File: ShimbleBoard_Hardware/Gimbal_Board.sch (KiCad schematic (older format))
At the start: 54 parts, among them Q1 2N3904, Q2 2N3904, Q3 2N3904, Q4 2N3904, Q5 2N3904, Q6 2N3904, Q7 2N3904, Q8 2N3904, U1 TM4C129E_Launchpad, U2 OKI, U3 OKI

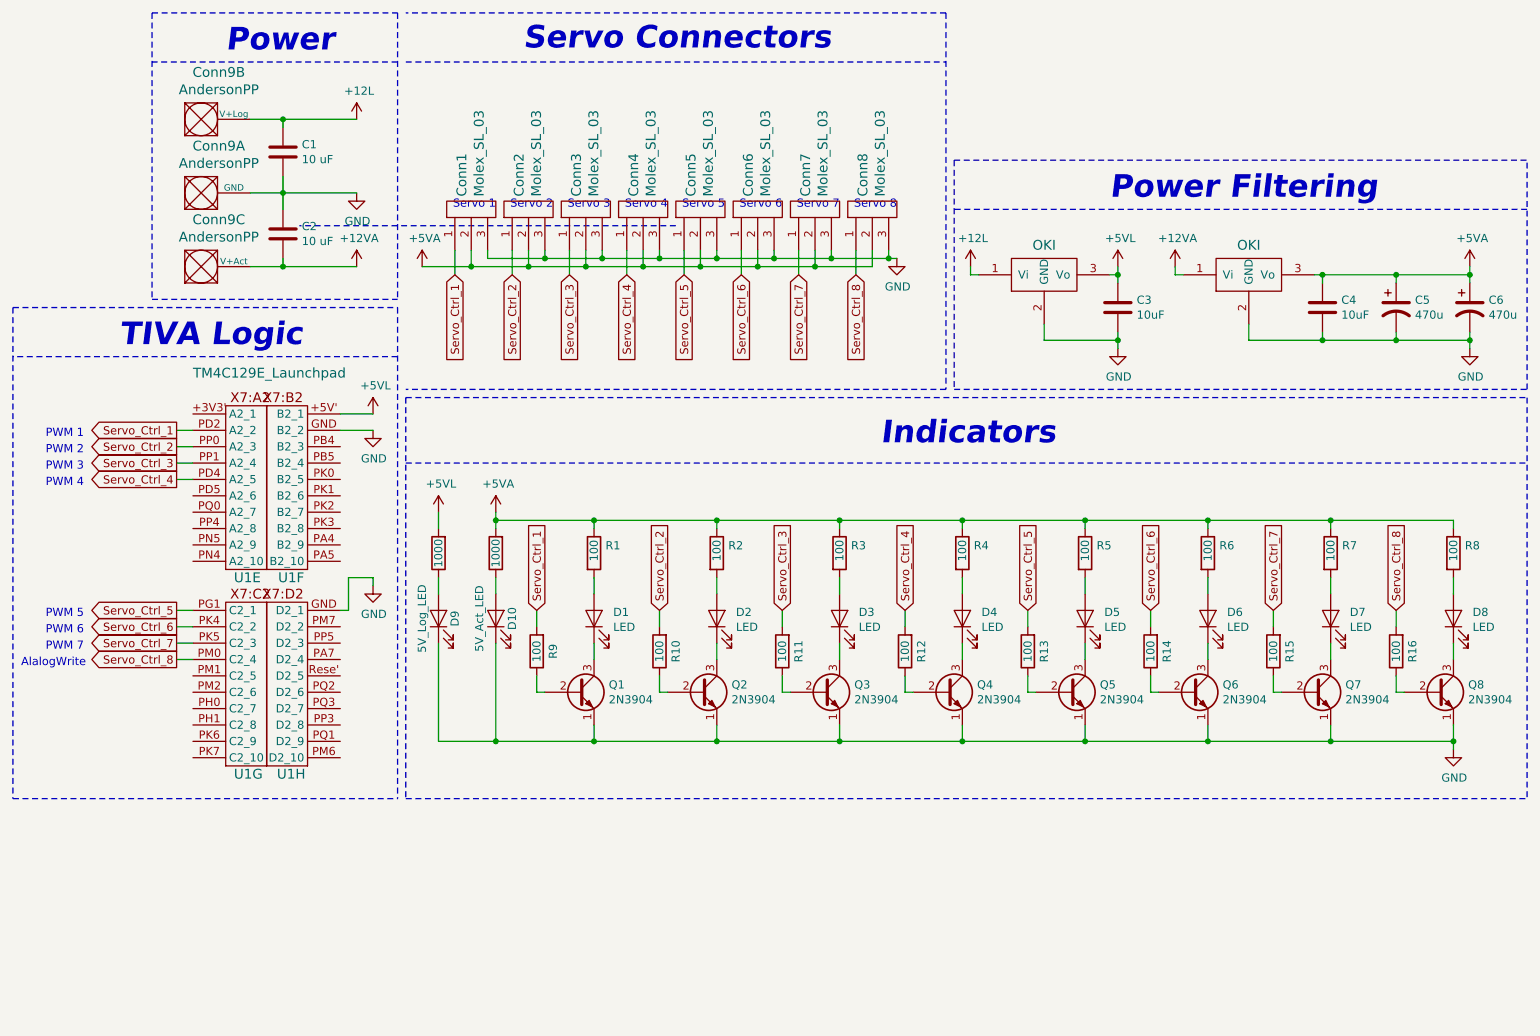
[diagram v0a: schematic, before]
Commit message: Noice
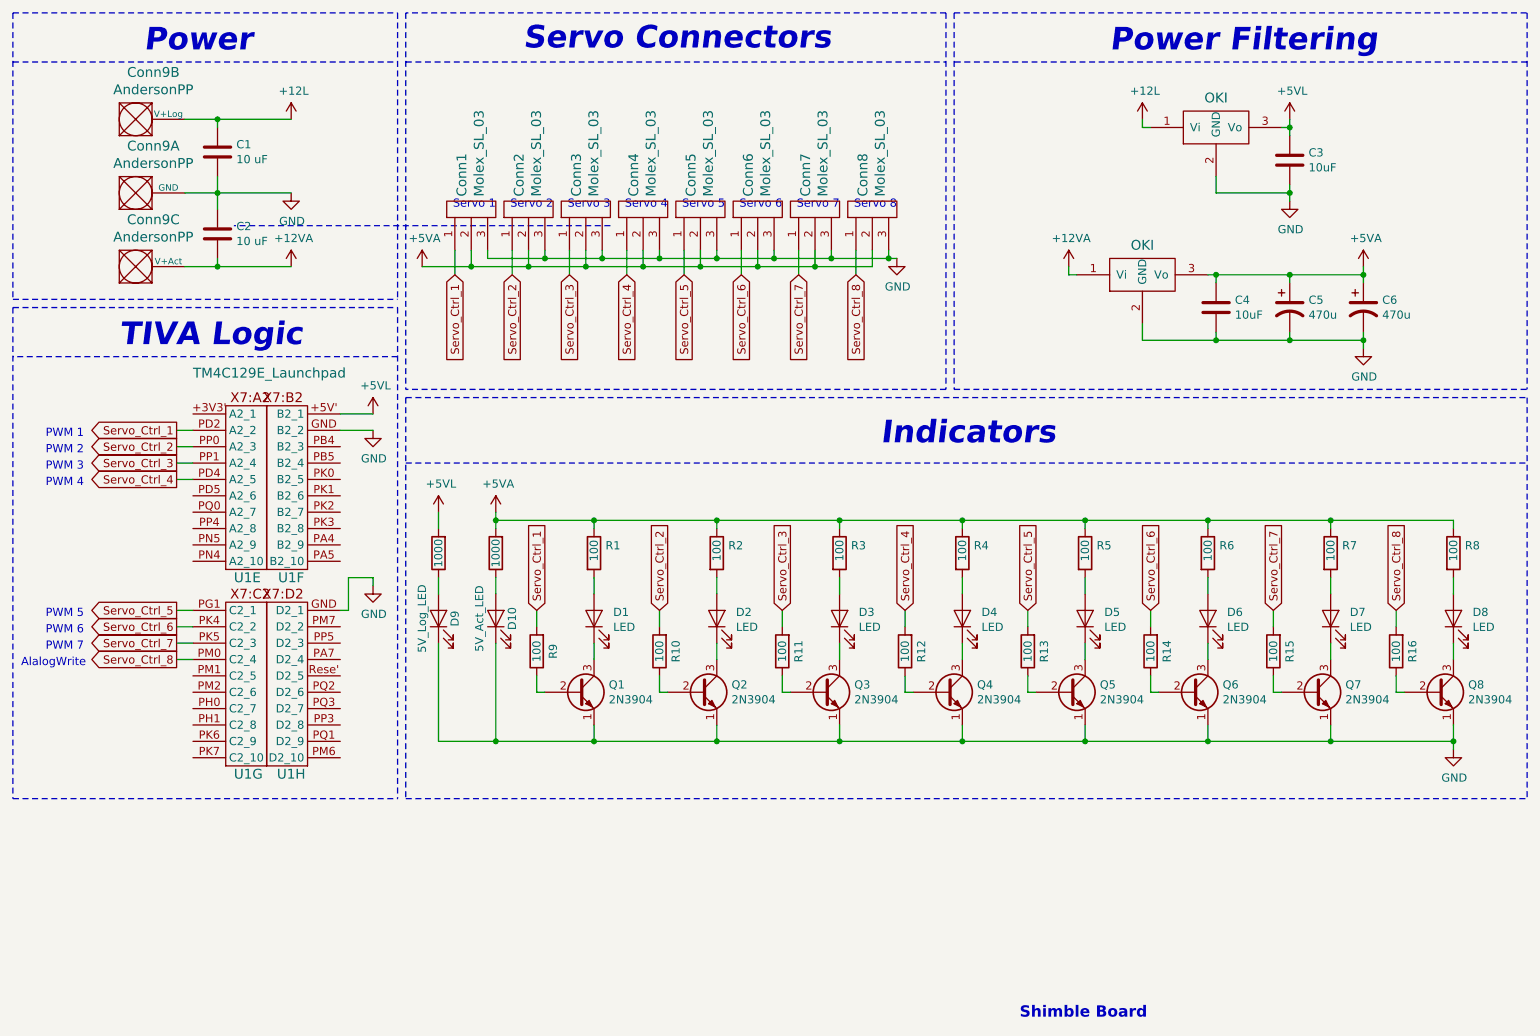
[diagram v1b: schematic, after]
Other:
- note added: "Shimble Board"
- moved on the sheet: C1, C2, C3, C4, C5, C6, Conn9A, Conn9B, Conn9C
